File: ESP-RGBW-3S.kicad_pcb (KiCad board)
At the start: 2 copper layers, 66.7 x 48.3 mm, 53 parts, among them J1 12V In, J2 PROG, J3 LED Str., J4 Temp. S., J5 Light. S., J6 PIR, J91 12V In, Q1 IRLML0040TRPBF, Q2 IRLML0040TRPBF, Q3 IRLML0040TRPBF, Q4 IRLML0040TRPBF, SW1 Flash, U2 ESP-12E, U4 DCDC_LM2596, U94 MP1584

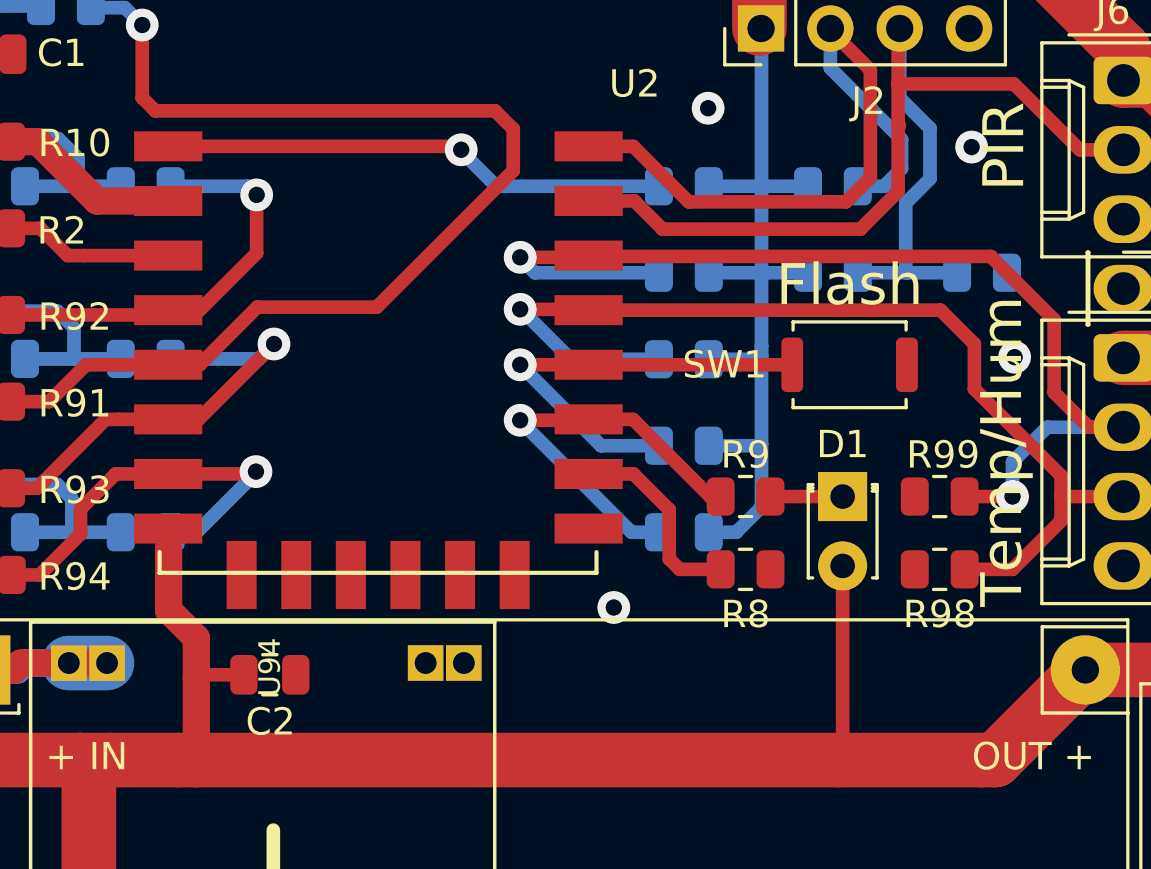
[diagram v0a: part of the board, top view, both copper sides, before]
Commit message: gerber files
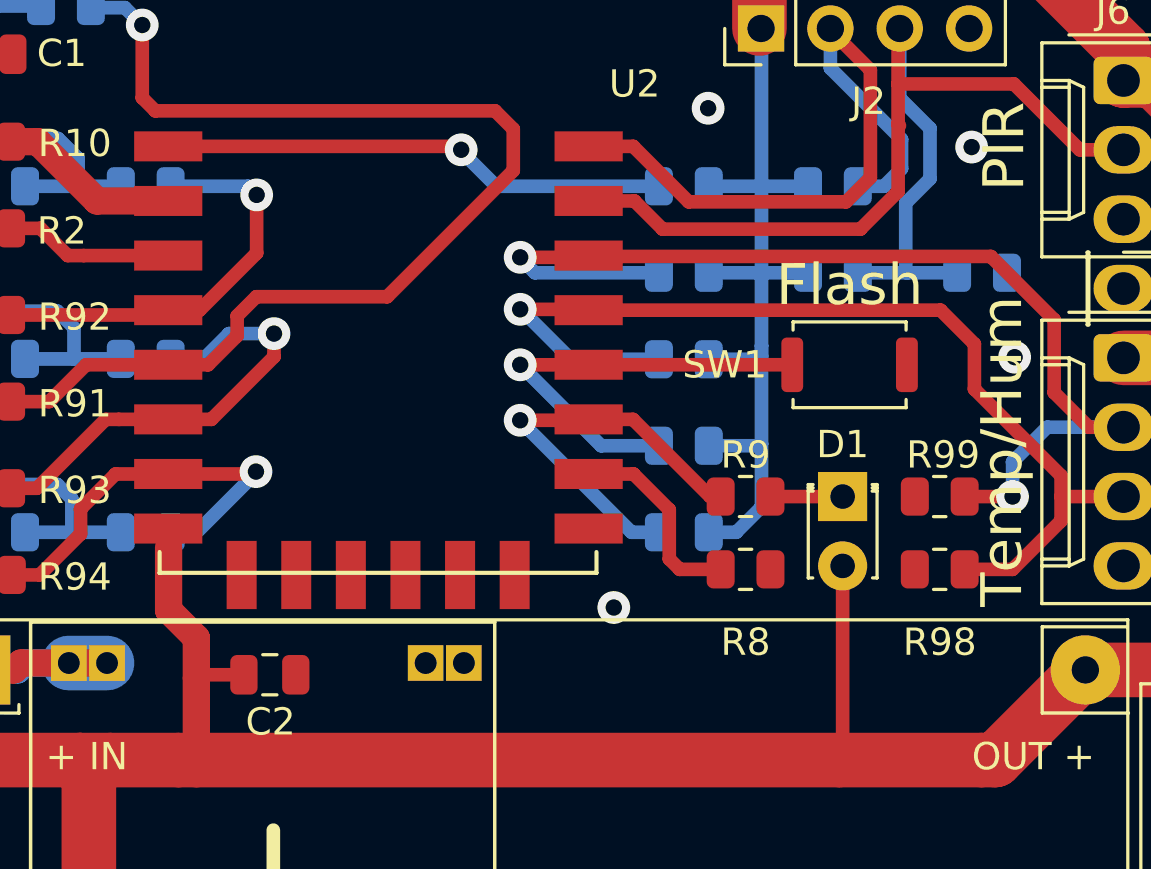
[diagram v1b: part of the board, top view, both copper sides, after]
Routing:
- net Blue: track 16.1 -> 17.0 mm

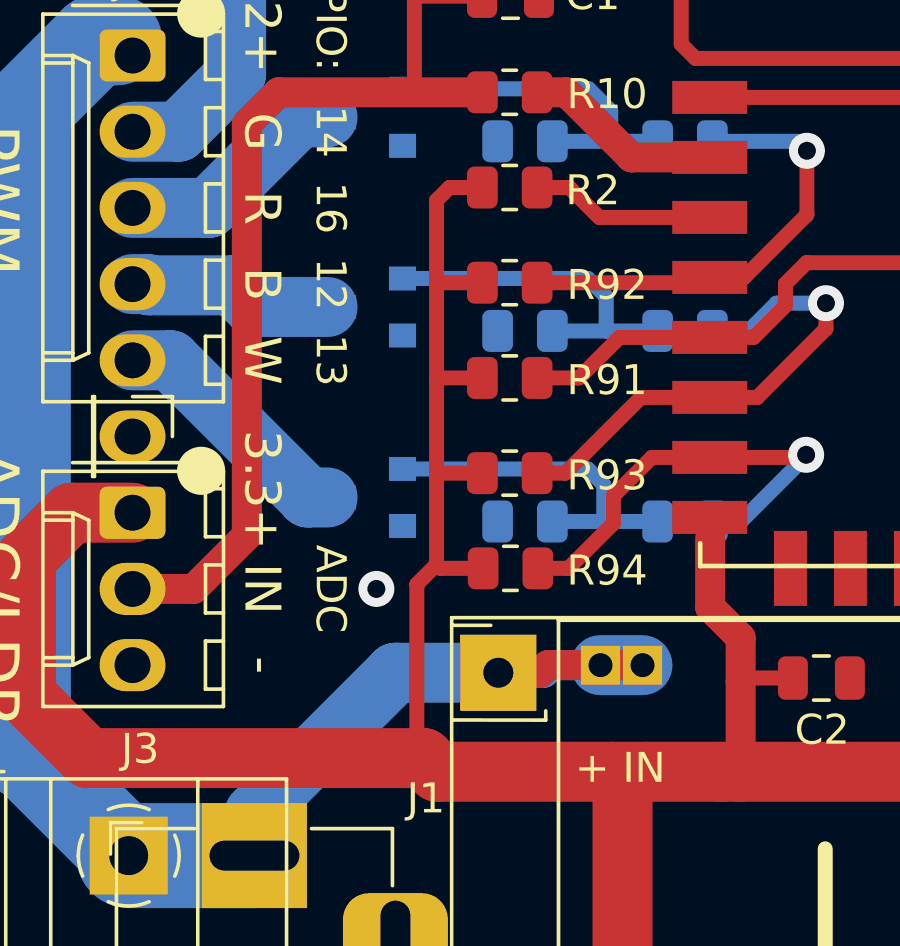
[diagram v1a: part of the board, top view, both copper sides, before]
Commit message: .
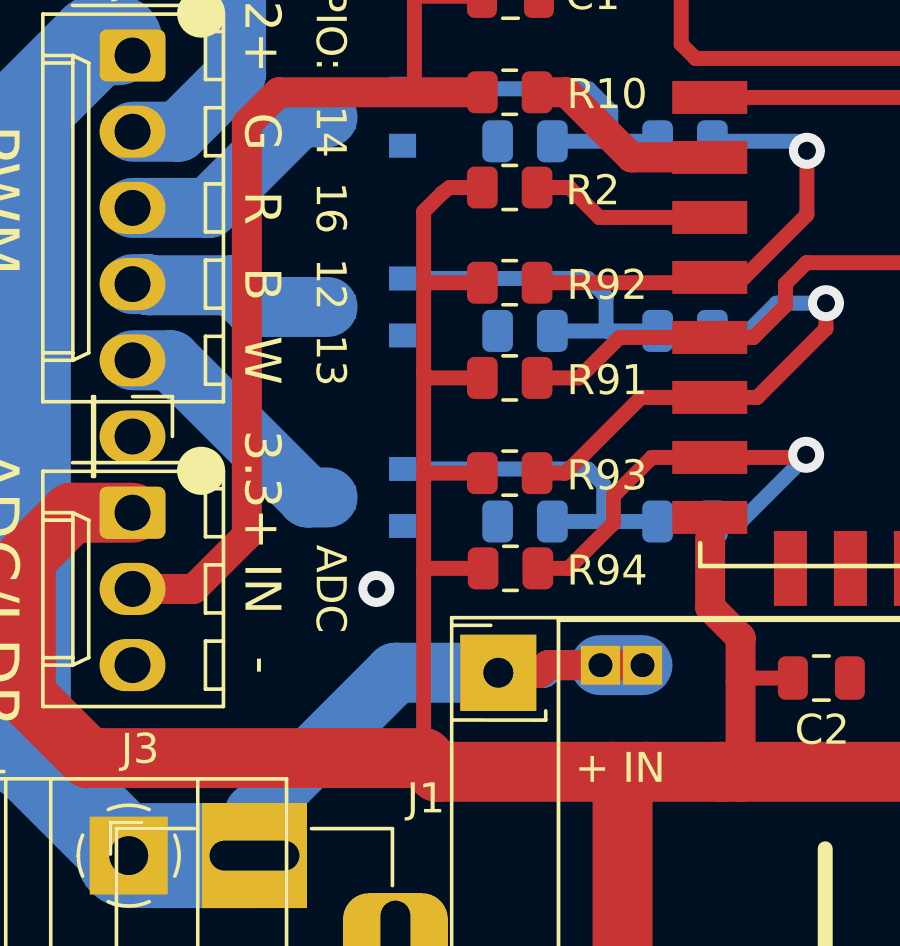
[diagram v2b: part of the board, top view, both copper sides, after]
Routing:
- net +3V3: track 213.9 -> 215.9 mm
